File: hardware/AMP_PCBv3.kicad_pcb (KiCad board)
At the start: 2 copper layers, 70 x 82.5 mm, 83 parts, among them CN1 Male_L1, CN2 Male_R2, J1 Input_PWR, J2 VESC_PPM, J3 VESC_COMM, J4 LED_Header, J5 USB_B_Mini, J6 STEERING, M1 Fan_PC_3pin, M2 Brake, M3 Fan_PC_3pin, M4 Fan_PC_3pin, M5 Fan_PC_3pin, Q1 DMN2310U, Q2 DMN2310U, Q3 DMN2310U, Q4 DMN2310U, U1 VNH7070AS, U10 SN74LVC1T45DCK, U11 SN74LVC1T45DCK, U2 AP64500, U3 USBLC6-2SC6, U4 TLV74318P, U5 ICM-20948, U6 FT230XS, U7 RFM95W-915S2, U8 SN74LVC1T45DCK, U9 SN74LVC1T45DCK

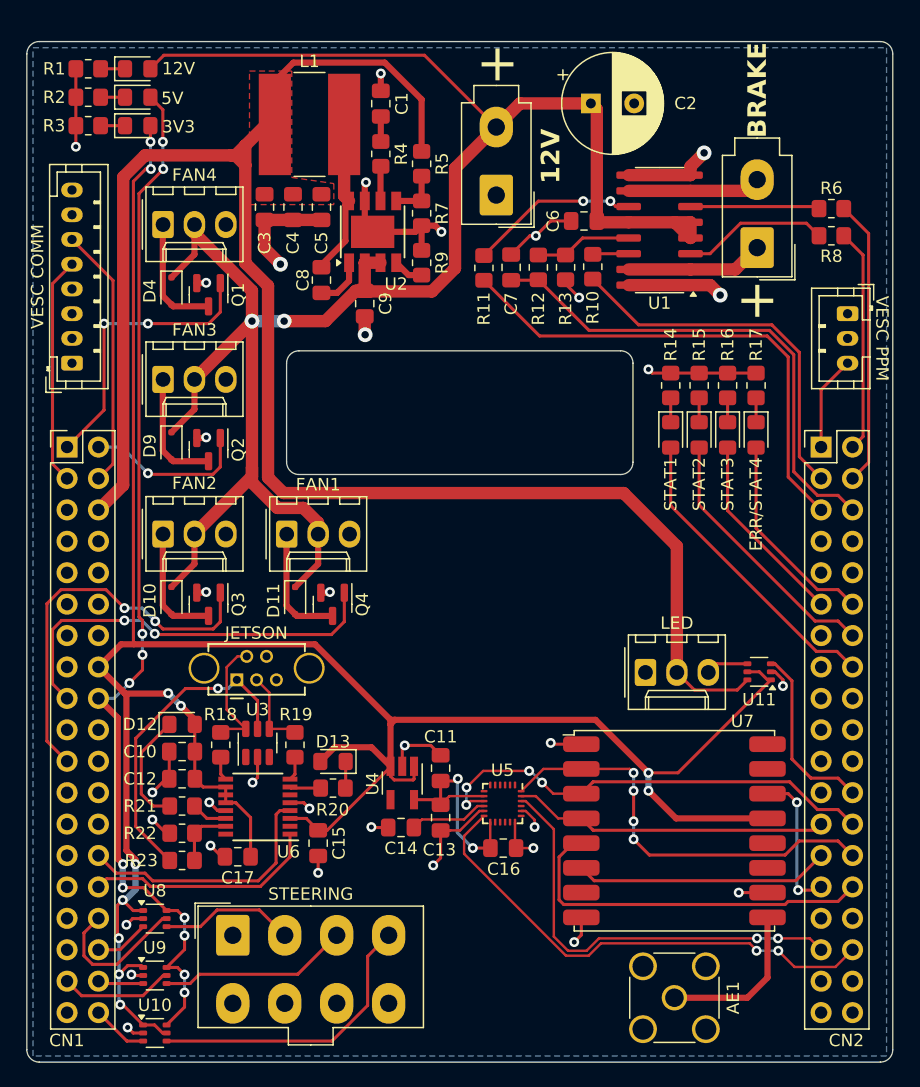
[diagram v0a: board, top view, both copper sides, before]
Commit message: Schematic cleanup
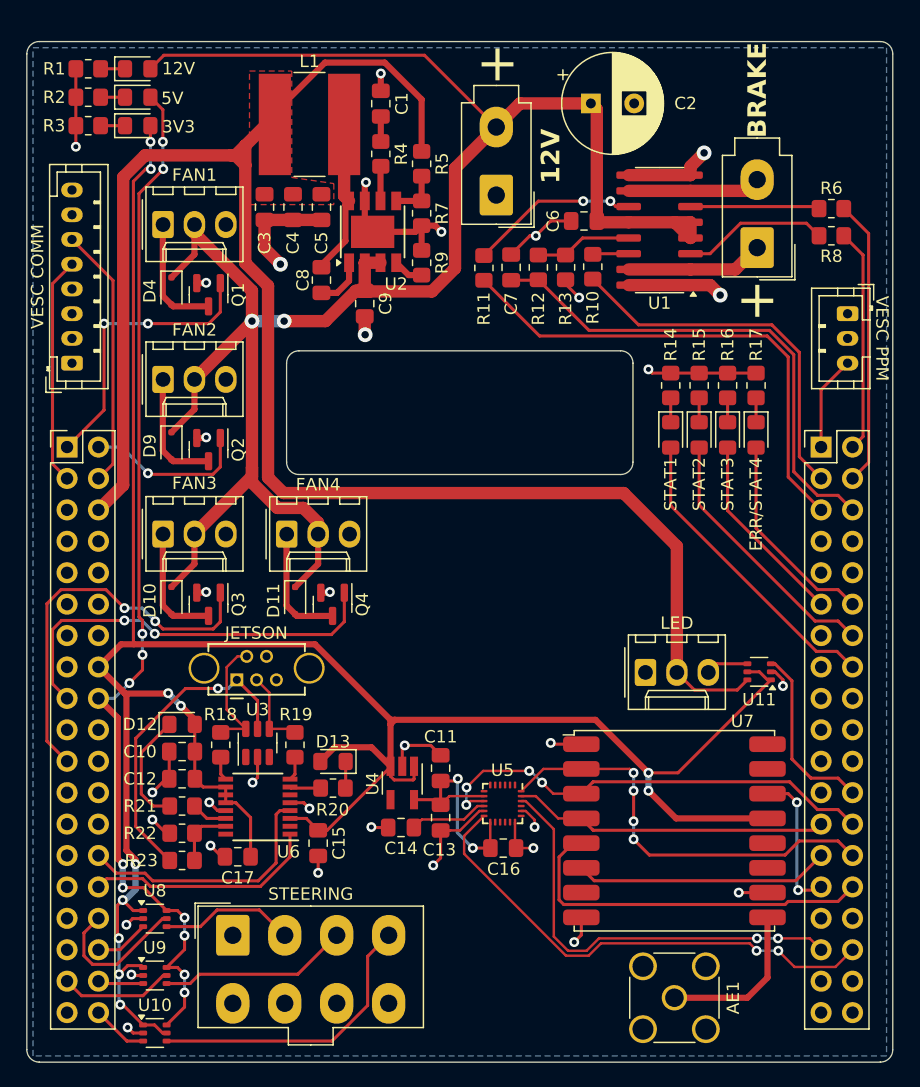
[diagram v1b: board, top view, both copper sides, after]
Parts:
- removed CN1: Male_L1, Connector_PinHeader_2.54mm:PinHeader_2x19_P2.54mm_Vertical
- removed CN2: Male_R2, Connector_PinHeader_2.54mm:PinHeader_2x19_P2.54mm_Vertical
- added U12: ~, AMP_Custom:NUCLEO64, F.Cu at (143.8, 78.5)
- D5: value STAT4 -> STAT1
- D6: value STAT3 -> STAT2
- D7: value STAT2 -> STAT3
- D8: value STAT1 -> STAT4
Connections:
- net /E5V renamed +5P
- net /LED_SIG_5V renamed /Status LEDs/LED_SIG_5V
- net /PB10 renamed /SPI2_SCK
- net /PB14 renamed /SPI2_MISO
- net /PB15 renamed /SPI2_MOSI
- net Net-(M2-+) renamed /Brake Controller/OUT_A
- net Net-(M2--) renamed /Brake Controller/OUT_B
- D5 pad 2: /PB12 -> /STAT1
- D6 pad 2: /PA11 -> /STAT2
- D7 pad 2: /PA5 -> /STAT3
- D8 pad 2: /PA12 -> /STAT4
- J2 pad 3: /PC9 -> /VESC_SERVO
- J3 pad 5: /PC12 -> /UART5_TX
- J3 pad 6: /PD2 -> /UART5_RX
- Q1 pad 1: /PC10 -> /FAN1
- Q2 pad 1: /PC11 -> /FAN2
- Q3 pad 1: /PB7 -> /FAN3
- Q4 pad 1: /PA15 -> /FAN4
- U10 pad 3: /PC0 -> /STEERING_ENABLE+_3V3
- U6 pad 1: /PA1 -> /UART4_RX
- U6 pad 4: /PA0 -> /UART4_TX
- U7 pad 14: /PB5 -> /LORA_DIO0
- U7 pad 5: /PB13 -> /LORA_NSS
- U7 pad 6: /PB4 -> /LORA_RST
- U8 pad 3: /PB0 -> /STEERING_INPUT_B+_3V3
- U8 pad 5: /PA4 -> /STEERING_INPUT_B+_DIR
- U9 pad 3: /PC1 -> /STEERING_INPUT_A+_3V3
- U9 pad 5: /PC2 -> /STEERING_INPUT_A+_DIR
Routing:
- net /PA15: track 33.2 -> 0.00 mm, vias 2 -> 0
- net /FAN4: track 0.00 -> 33.2 mm, vias 0 -> 2
- net /PB7: track 31.8 -> 0.00 mm, vias 2 -> 0
- net /FAN3: track 0.00 -> 31.8 mm, vias 0 -> 2
- net /PB13: track 30.2 -> 0.00 mm
- net /LORA_NSS: track 0.00 -> 30.2 mm
- net /STAT1: track 0.00 -> 24.8 mm
- net /PB12: track 24.8 -> 0.00 mm
- net /PC10: track 23.3 -> 0.00 mm, vias 2 -> 0
- net /FAN1: track 0.00 -> 23.3 mm, vias 0 -> 2
- net /STAT2: track 0.00 -> 21.4 mm
- net /PA11: track 21.4 -> 0.00 mm
- net /UART5_RX: track 0.00 -> 21.2 mm
- net /PD2: track 21.2 -> 0.00 mm
- net /UART4_TX: track 0.00 -> 21.0 mm
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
